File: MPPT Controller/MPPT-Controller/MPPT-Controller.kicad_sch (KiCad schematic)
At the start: 1 part, among them U1 ADS1115IDGS

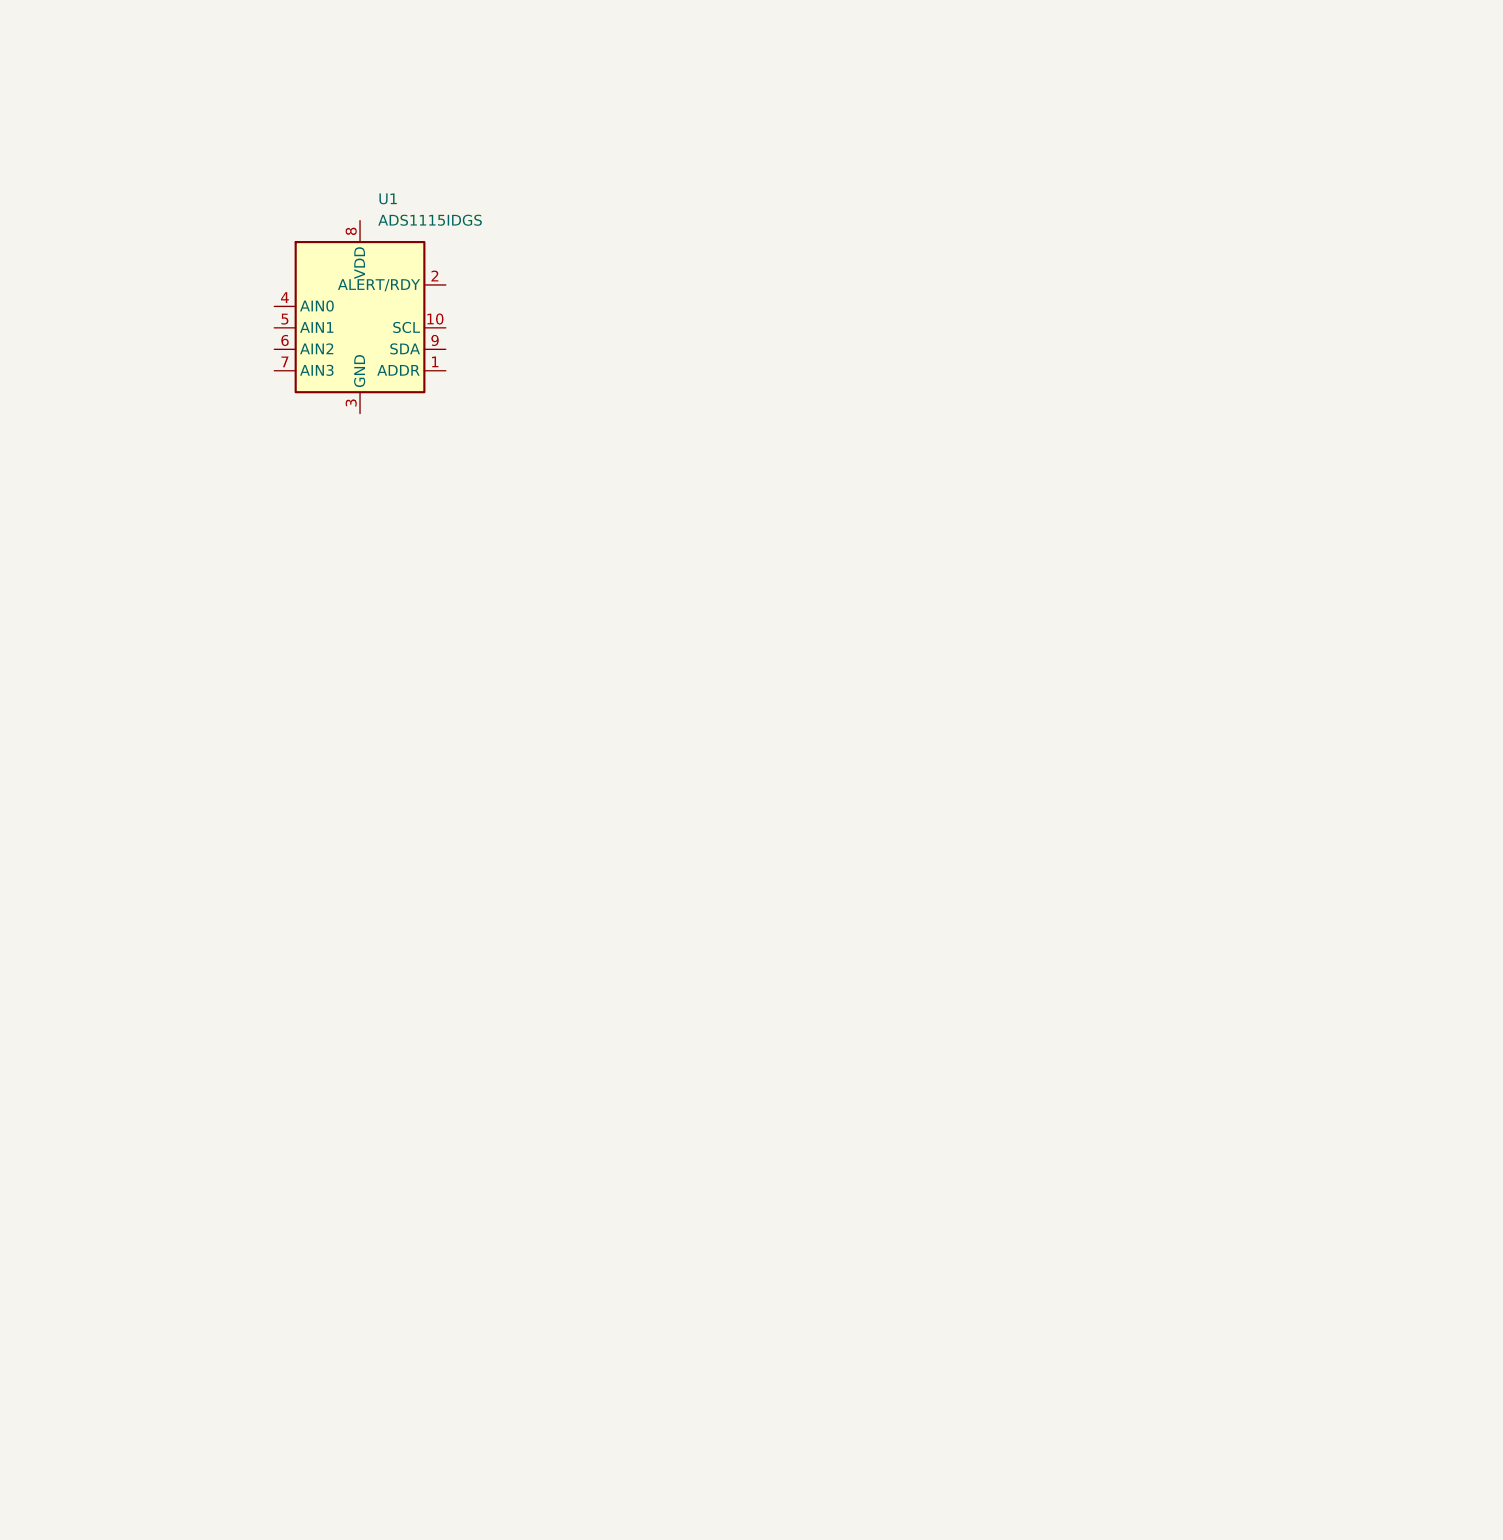
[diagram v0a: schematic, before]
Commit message: Update
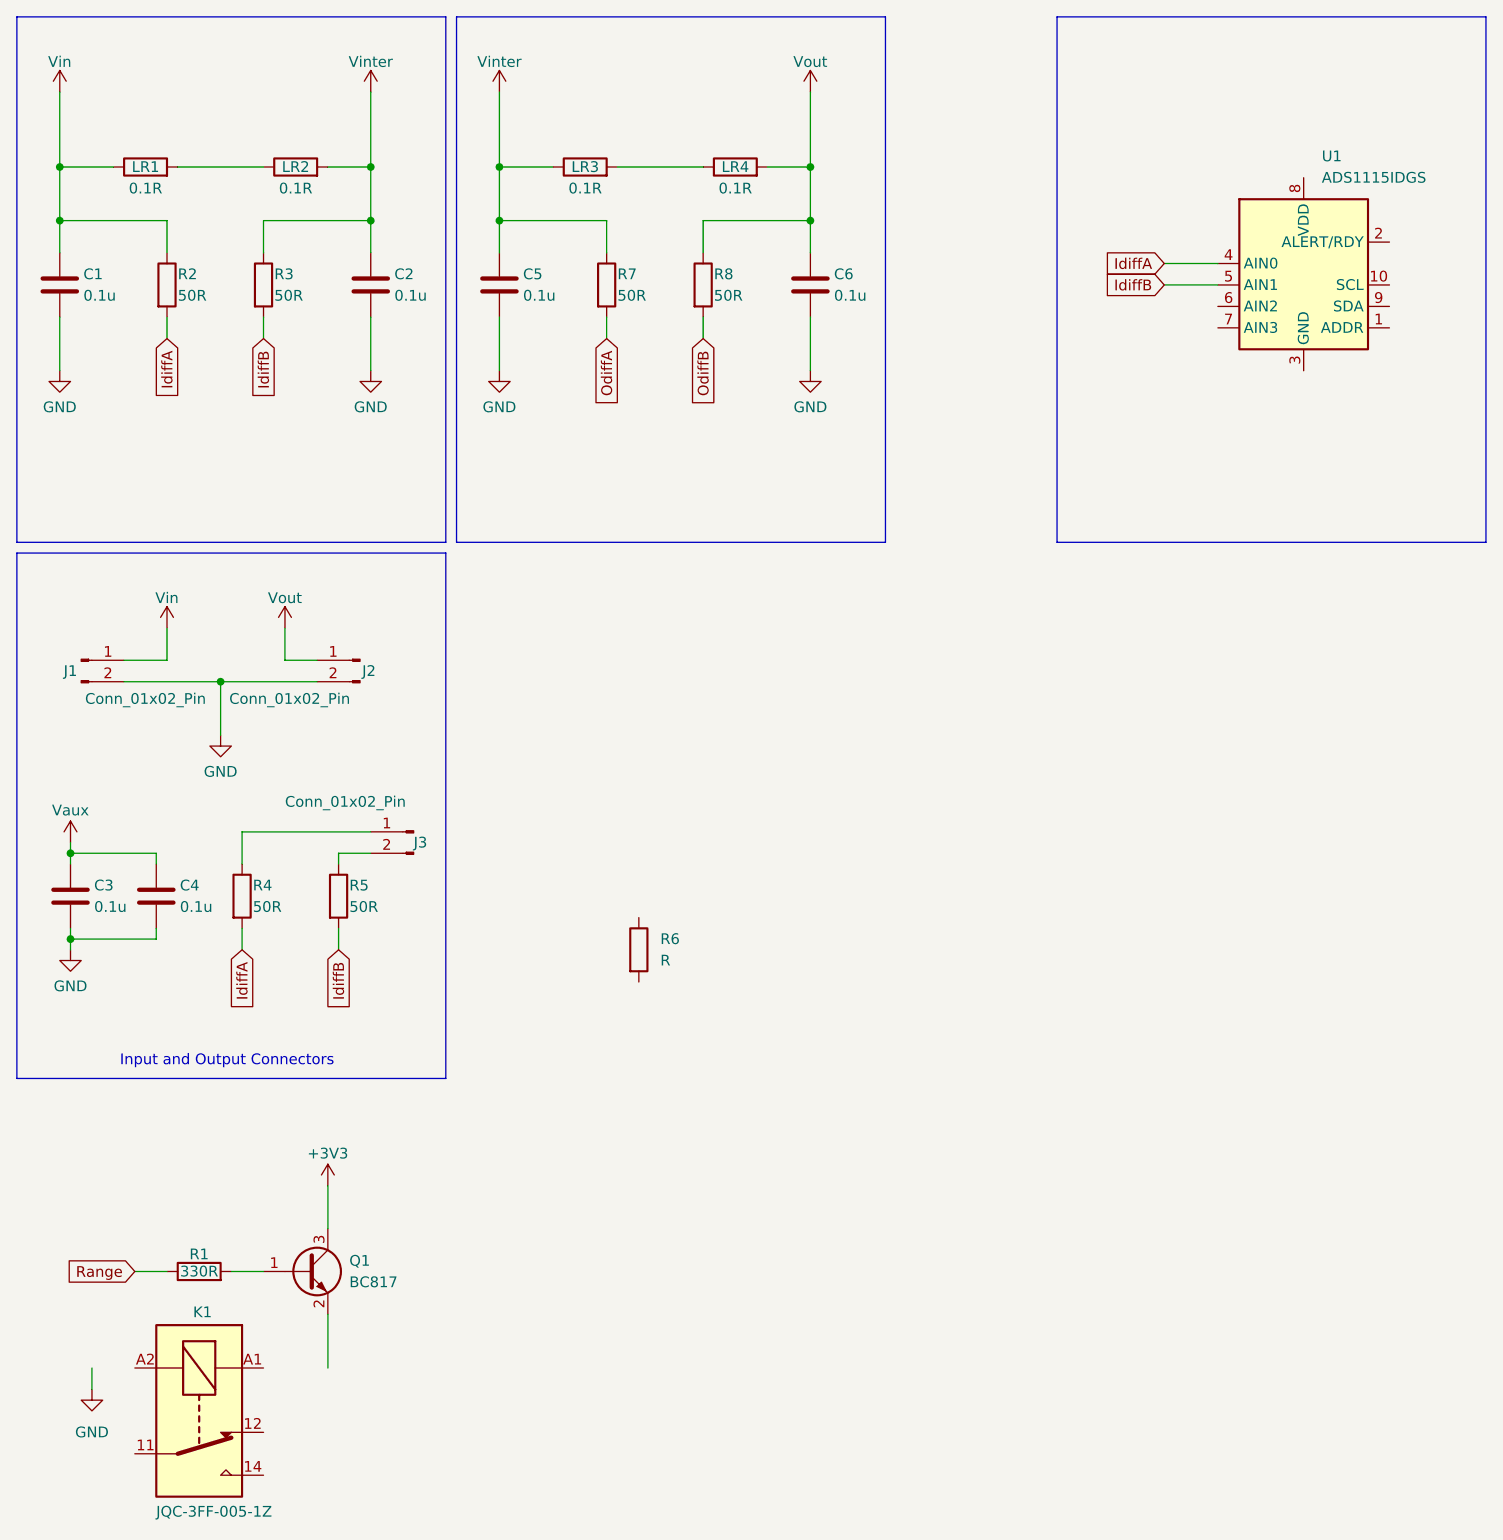
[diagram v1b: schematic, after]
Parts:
- added C1, C2, C3, C4, C5, C6: 0.1u, Capacitor_SMD:C_0603_1608Metric_Pad1.08x0.95mm_HandSolder, symbol Device:C
- added J1, J2, J3: Conn_01x02_Pin, symbol Connector:Conn_01x02_Pin
- added K1: JQC-3FF-005-1Z, Relay_THT:Relay_SPDT_Hongfa_JQC-3FF_0XX-1Z, symbol Relay:JQC-3FF-005-1Z
- added LR1, LR2, LR3, LR4: 0.1R, symbol Device:R
- added Q1: BC817, Package_TO_SOT_SMD:SOT-23_Handsoldering, symbol Transistor_BJT:BC817
- added R1: 330R, Resistor_SMD:R_0603_1608Metric_Pad0.98x0.95mm_HandSolder, symbol Device:R
- added R2, R3, R4, R5, R7, R8: 50R, symbol Device:R
- added R6: R, symbol Device:R
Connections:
- net IdiffA: now reaches U1.4 (AIN0)
- net IdiffA: now also R2.2, R4.2
- net IdiffB: now reaches U1.5 (AIN1)
- net IdiffB: now also R3.2, R5.2
- new net: Q1.1 (B), R1.2
- new net: LR3.2, LR4.1
- new net: LR1.2, LR2.1
- new net: J3.2 (Pin_2), R5.1
- new net: J3.1 (Pin_1), R4.1
- new net +3V3: Q1.3 (C)
- new net GND: C1.2, C2.2, C3.2, C4.2, C5.2, C6.2, J1.2 (Pin_2), J2.2 (Pin_2)
- new net OdiffA: R7.2
- new net OdiffB: R8.2
- new net Range: R1.1
- new net Vaux: C3.1, C4.1
- new net Vin: C1.1, J1.1 (Pin_1), LR1.1, R2.1
- new net Vinter: C2.1, C5.1, LR2.2, LR3.1, R3.1, R7.1
- new net Vout: C6.1, J2.1 (Pin_1), LR4.2, R8.1
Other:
- note added: "Input and Output Connectors"
- moved on the sheet: U1
